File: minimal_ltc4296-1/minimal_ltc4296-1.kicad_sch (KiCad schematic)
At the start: 2 parts, among them U1 LTC4296AUK-1-PBF

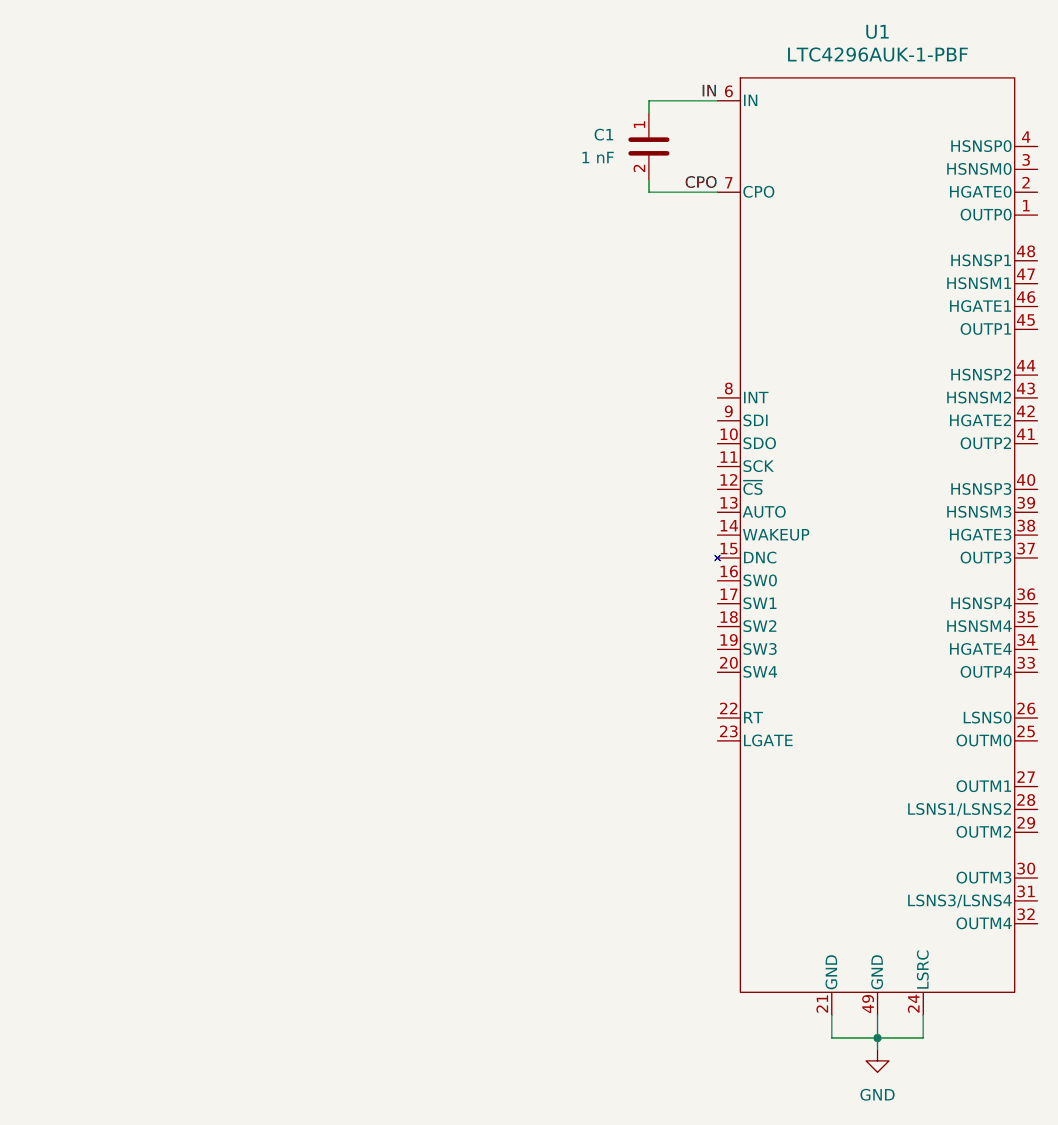
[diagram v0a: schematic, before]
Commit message: Update KiCAD files and submodule
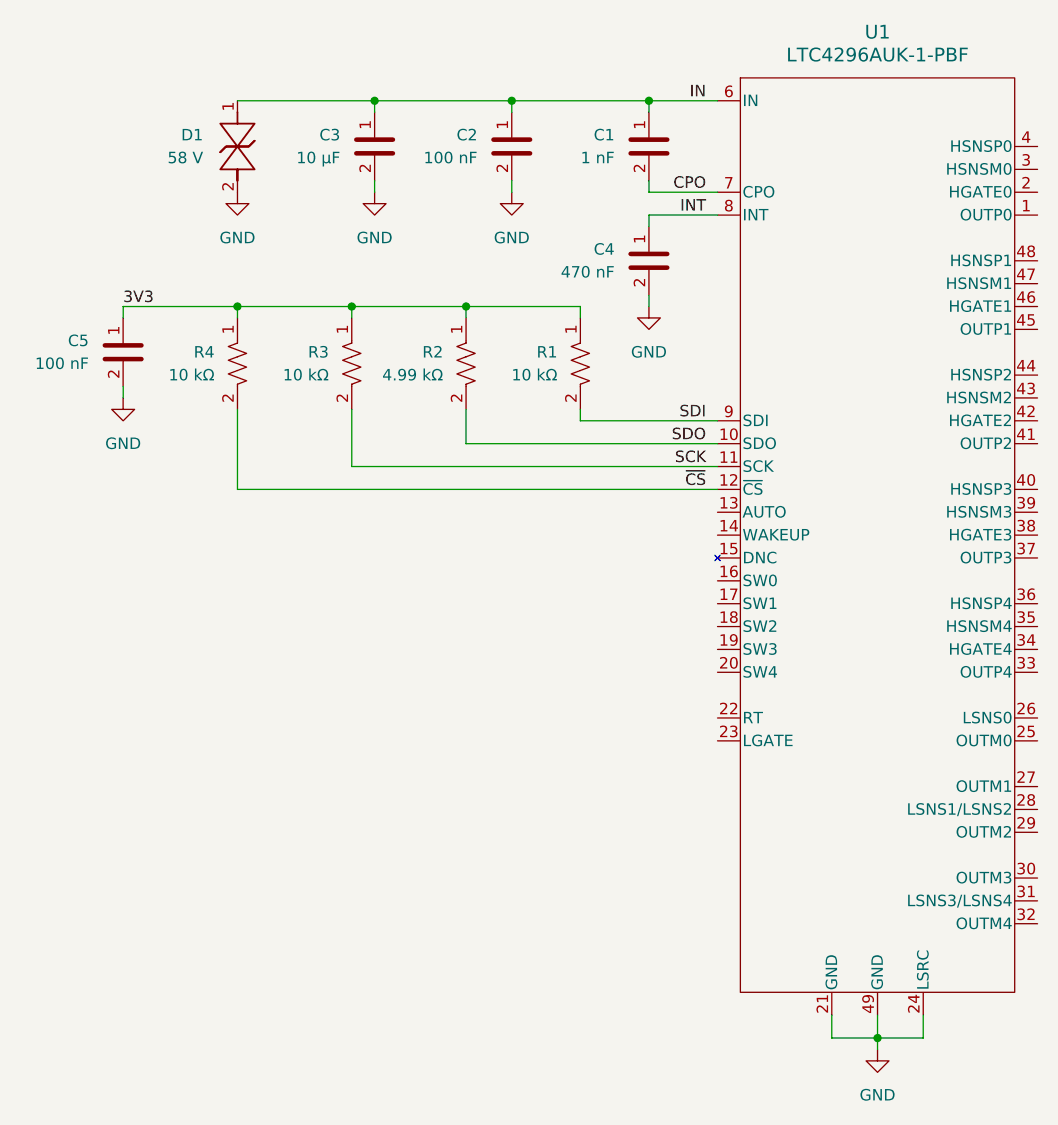
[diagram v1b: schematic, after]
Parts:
- added C2, C5: 100 nF, capacitor_footprints:C_0603_1608Metric, symbol CAPACITORS_C1608X7S2A_DATA_BASE:C_C1608X7S2A104K080AB
- added C3: 10 µF, capacitor_footprints:C_1210_250_3225Metric, symbol CAPACITORS_GRM32EC72A_DATA_BASE:C_GRM32EC72A106KE05L
- added C4: 470 nF, capacitor_footprints:C_0402_1005Metric, symbol CAPACITORS_C1005X5R1E_DATA_BASE:C_C1005X5R1E474K050BB
- added D1: 58 V, diode_footprints:DO-214AA, symbol DIODES_SMBJ_DATA_BASE:D_SMBJ58CA
- added R1, R3, R4: 10 kΩ, resistor_footprints:R_0402_1005Metric, symbol RESISTORS_ERJ-2RKF_DATA_BASE:R_ERJ-2RKF1002X
- added R2: 4.99 kΩ, resistor_footprints:R_0402_1005Metric, symbol RESISTORS_ERJ-2RKF_DATA_BASE:R_ERJ-2RKF4991X
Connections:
- net GND: now also C2.2, C3.2, C4.2, C5.2, D1.2
- net IN: now also C2.1, C3.1, D1.1
- net SDO: now reaches U1.10 (SDO)
- net SDO: now also R2.2
- net SCK: now reaches U1.11 (SCK)
- net SCK: now also R3.2
- net ~{CS}: now reaches U1.12 (~{CS})
- net ~{CS}: now also R4.2
- net INT: now reaches U1.8 (INT)
- net INT: now also C4.1
- net SDI: now reaches U1.9 (SDI)
- net SDI: now also R1.2
- new net 3V3: C5.1, R1.1, R2.1, R3.1, R4.1
